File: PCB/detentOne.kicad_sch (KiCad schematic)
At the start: 0 parts

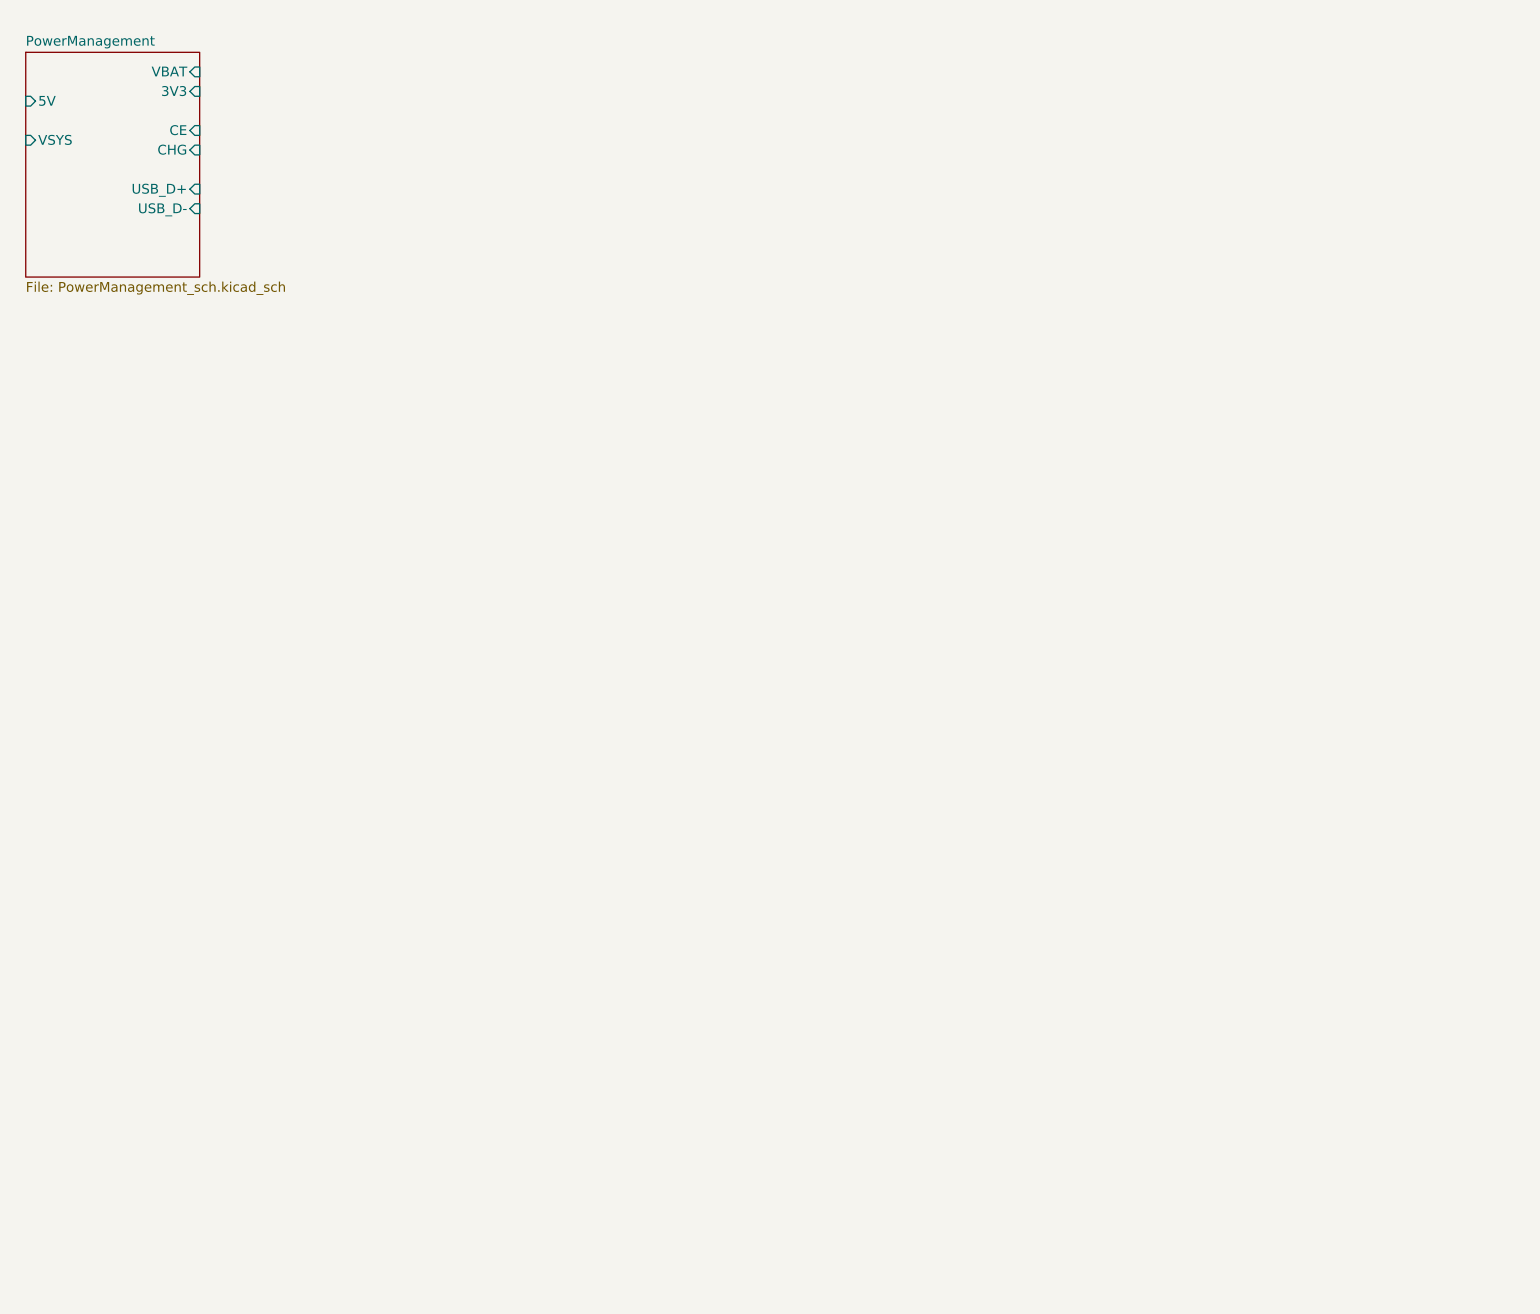
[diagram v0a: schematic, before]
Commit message: Adding microSD
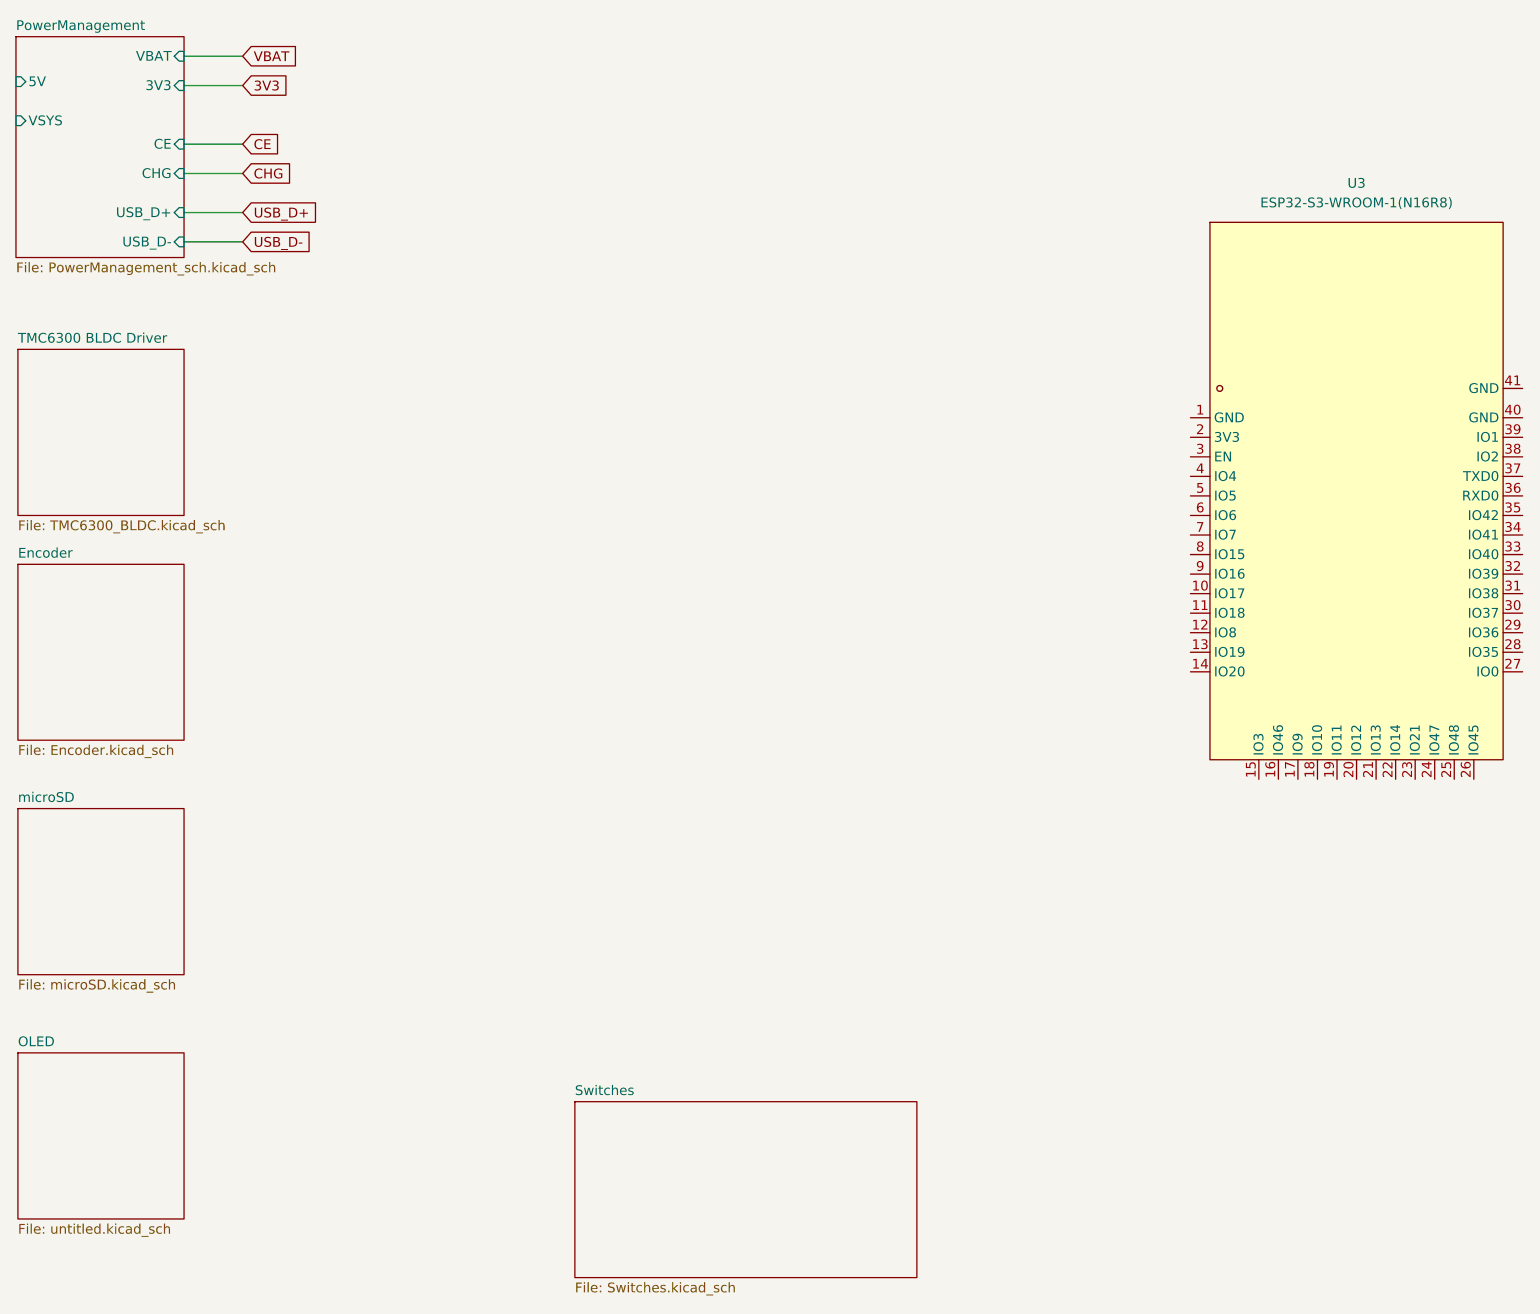
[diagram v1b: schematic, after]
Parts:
- added U3: ESP32-S3-WROOM-1(N16R8), easyeda2kicad:WIRELM-SMD_ESP32-S3-WROOM-1, symbol easyeda2kicad:ESP32-S3-WROOM-1(N16R8)
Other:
- added sheet Encoder (Encoder.kicad_sch)
- added sheet OLED (untitled.kicad_sch)
- added sheet Switches (Switches.kicad_sch)
- added sheet TMC6300 BLDC Driver (TMC6300_BLDC.kicad_sch)
- added sheet microSD (microSD.kicad_sch)
